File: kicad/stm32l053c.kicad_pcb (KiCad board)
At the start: 2 copper layers, 52 x 35 mm, 43 parts, among them P1 SWD, P2 PWR, Q1 BC807, Q2 BC817, SW1 SW_PUSH, SW2 SW_PUSH, SW3 SW_PUSH, SW4 SW_SPDT, U1 STM32L053C8_LQFP48, U2 TLV61225, U3 um66t, Y1 Crystal_GND23

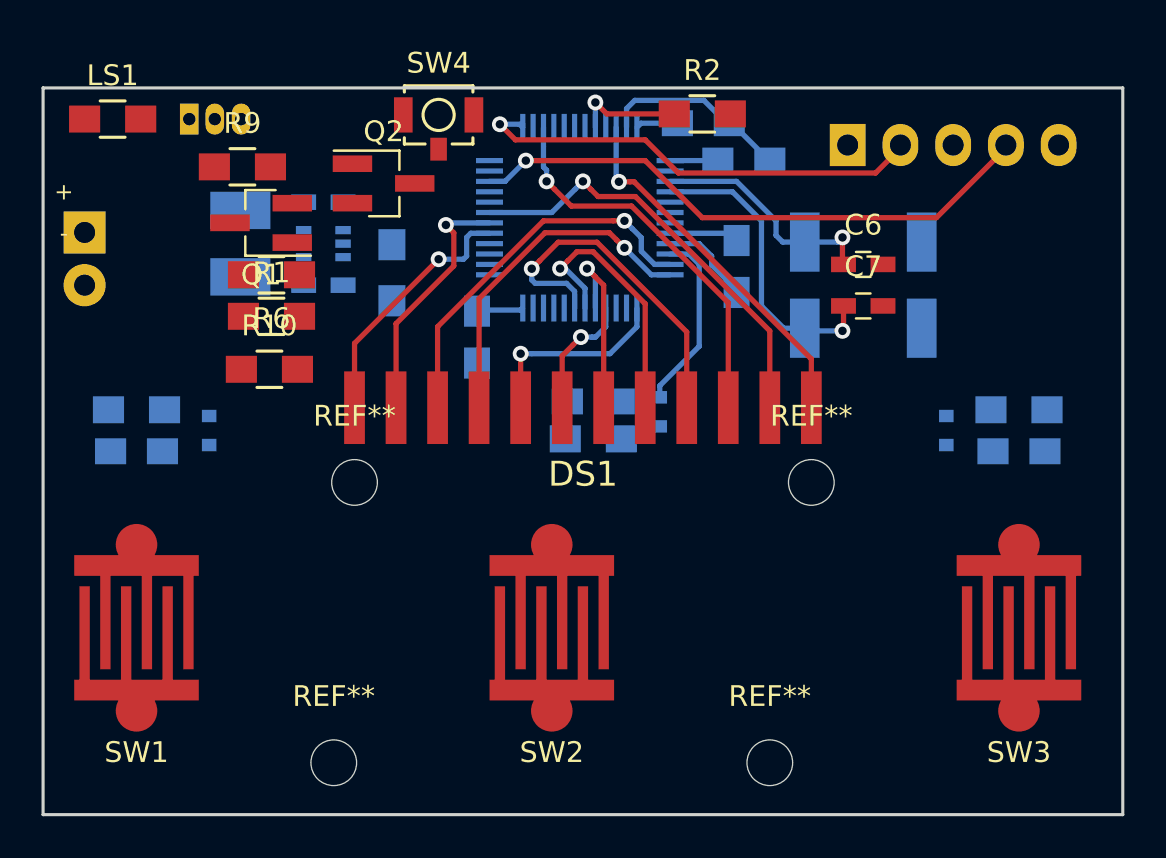
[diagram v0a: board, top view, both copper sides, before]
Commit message: Bottom initial routing
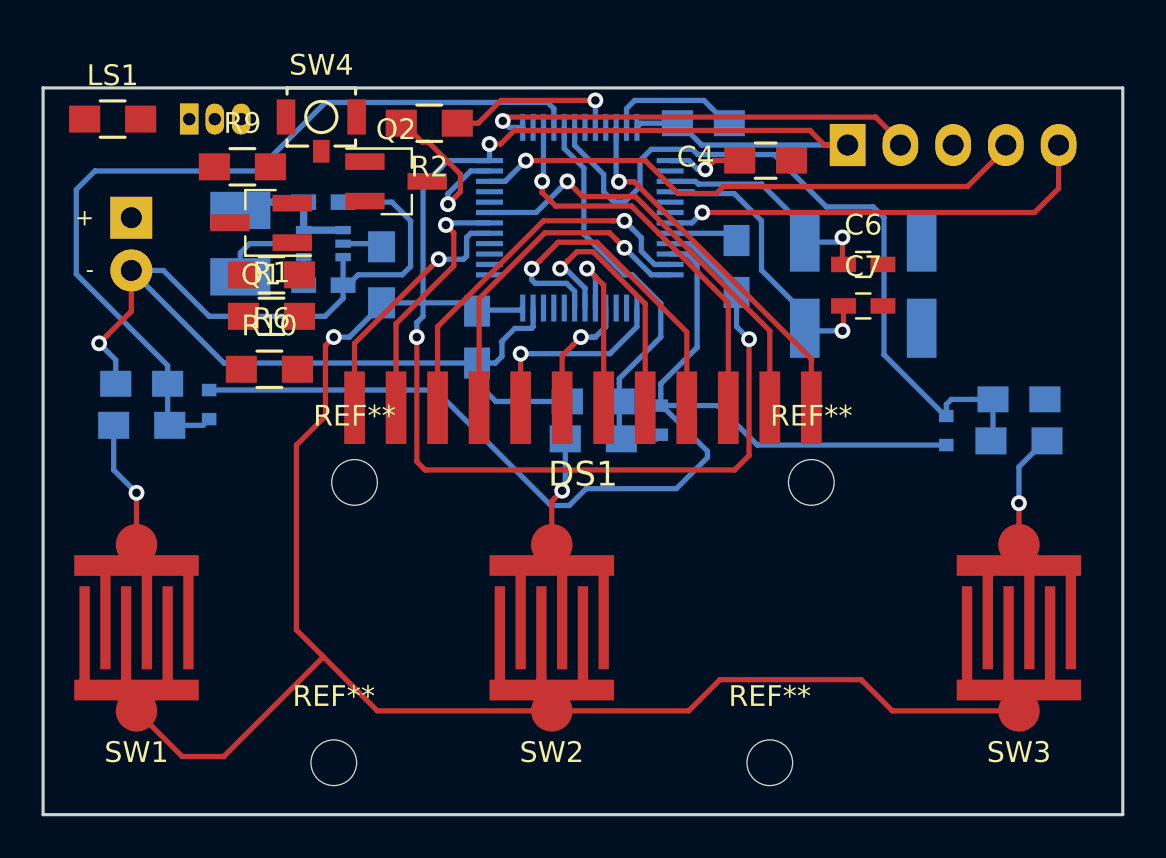
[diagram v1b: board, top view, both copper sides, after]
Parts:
- C4: moved to F.Cu
- moved R2 13.2 mm to (135.6, 87.3), turned to 180 degrees
- moved SW4 5.65 mm to (130.4, 87.0)
- moved C5 3.26 mm to (121.8, 99.8)
- moved C11 2.50 mm to (164.0, 100.6)
- moved P2 2.36 mm to (121.2, 91.8)
- moved R5 1.50 mm to (164.0, 102.6)
- moved D1 1.25 mm to (125.0, 100.8)
- moved C4 1.05 mm to (151.8, 89.1)
- moved R3 0.79 mm to (121.8, 101.8)
- moved Q2 0.61 mm to (134.0, 90.1)
- moved R7 0.51 mm to (133.3, 94.6)
- moved D2 0.40 mm to (146.8, 101.6)
- turned D3 to 90 degrees
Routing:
- net VDD: track 8.72 -> 150.8 mm, vias 0 -> 4
- net Earth: track 12.5 -> 77.0 mm, vias 0 -> 2
- net /WAKEUP_PIN1: track 8.80 -> 54.3 mm
- net /BUTTON0: track 0.00 -> 41.0 mm
- net /BUTTON2: track 0.00 -> 36.3 mm
- net NRST: track 0.00 -> 21.5 mm, vias 0 -> 1
- net /BUTTON1: track 0.00 -> 20.0 mm
- net +BATT: track 0.00 -> 6.47 mm
- net Net-(R3-Pad2): track 0.00 -> 6.21 mm, vias 0 -> 1
- net Net-(R5-Pad2): track 0.00 -> 5.62 mm, vias 0 -> 1
- net Net-(R4-Pad2): track 0.00 -> 5.37 mm, vias 0 -> 1
- net Net-(L1-Pad2): track 0.00 -> 4.39 mm
- net Net-(C8-Pad1): track 0.00 -> 3.26 mm
- net Net-(R2-Pad1): track 5.23 -> 8.41 mm
- net /VLCD: track 2.30 -> 3.82 mm, vias 0 -> 1
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- added copper zone on B.Cu, net Earth
